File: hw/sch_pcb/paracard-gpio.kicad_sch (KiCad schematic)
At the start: 1 part, among them P1 BTH-030-01-F-D-A

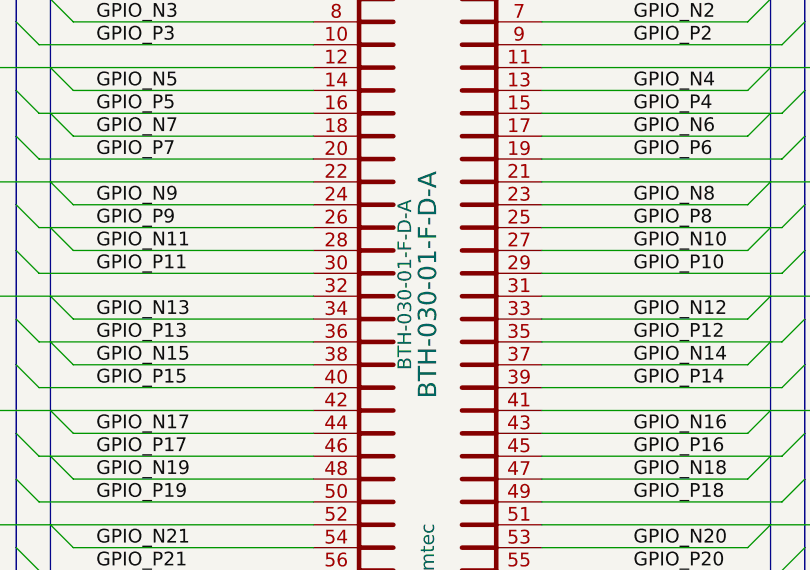
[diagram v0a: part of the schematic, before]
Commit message: Priprava pro osazeni
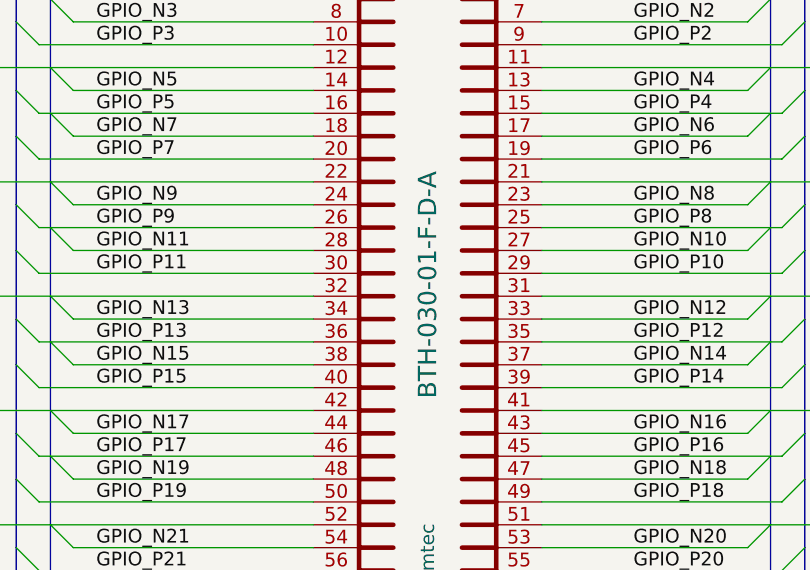
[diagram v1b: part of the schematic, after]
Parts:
- P1: value BTH-030-01-F-D-A -> (none); footprint Mlab_CON:SAMTEC-BTH-030-01-X-D-A -> (none); UST_ID (none) -> 628e4f00243ef5997b12f43c
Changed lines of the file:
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@@
       (effects (font (size 1.524 1.524)))
     )
-    (property "Value" "BTH-030-01-F-D-A" (id 1) (at 183.515 103.505 90)
+    (property "Value" "" (id 1) (at 183.515 103.505 90)
       (effects (font (size 1.524 1.524)))
     )
-    (property "Footprint" "Mlab_CON:SAMTEC-BTH-030-01-X-D-A" (id 2) (at 188.595 103.505 90)
+    (property "Footprint" "" (id 2) (at 188.595 103.505 90)
       (effects (font (size 1.524 1.524)) hide)
     )
@@
       (effects (font (size 1.524 1.524)))
     )
+    (property "UST_ID" "628e4f00243ef5997b12f43c" (id 6) (at 186.055 103.505 0)
+      (effects (font (size 1.27 1.27)) hide)
+    )
     (pin "1")

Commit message: update assets, save as 7
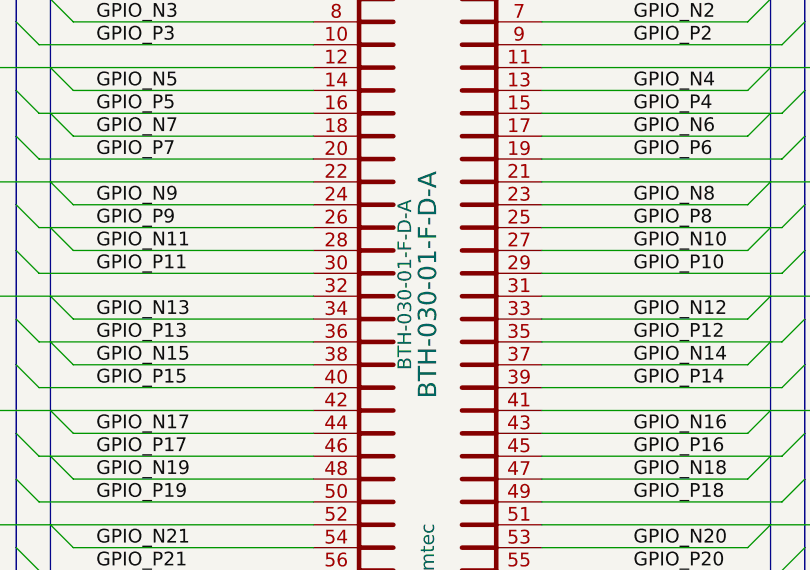
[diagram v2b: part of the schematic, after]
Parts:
- P1: value (none) -> BTH-030-01-F-D-A; footprint (none) -> Mlab_CON:SAMTEC-BTH-030-01-X-D-A
